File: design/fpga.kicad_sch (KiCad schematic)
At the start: 80 parts, among them J7 DEBUG_FPGA_GPIO, J8 DIGILENT_JTAG_HS2_01X06, SW1 RST, SW2 PROG, U13 XC7S15-FTGB196, U14 IS25LP064A-JKx

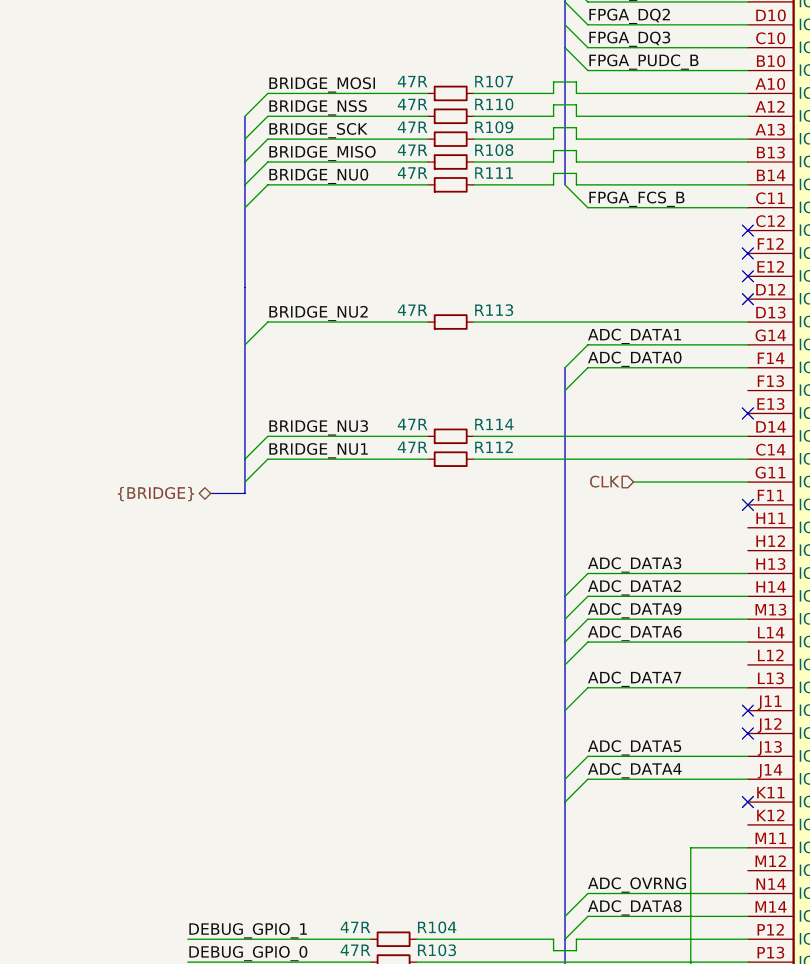
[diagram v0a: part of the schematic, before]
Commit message: Small layout update
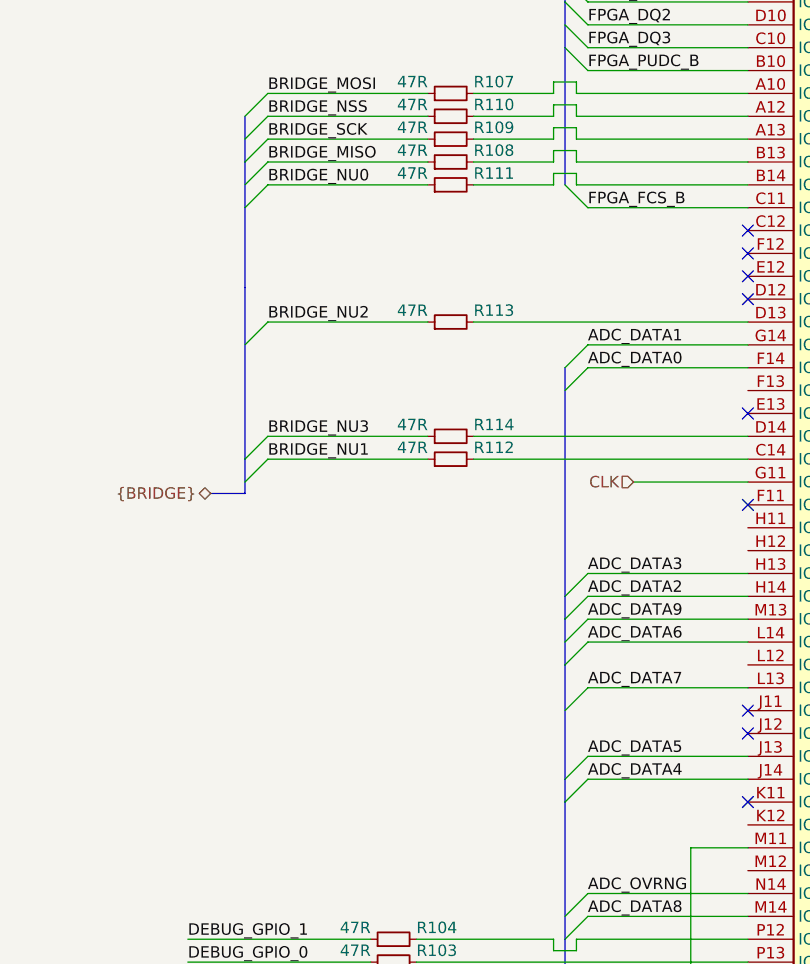
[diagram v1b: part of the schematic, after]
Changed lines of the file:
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@@
   (bus (pts (xy 125.73 85.09) (xy 129.54 85.09)))
   (bus (pts (xy 129.54 43.18) (xy 129.54 48.26)))
-  (bus (pts (xy 129.54 48.26) (xy 129.54 50.8)))
-  (bus (pts (xy 129.54 50.8) (xy 129.54 62.23)))
+  (bus (pts (xy 129.54 48.26) (xy 129.54 53.34)))
+  (bus (pts (xy 129.54 53.34) (xy 129.54 62.23)))
   (bus (pts (xy 129.54 62.23) (xy 129.54 81.28)))
   (bus (pts (xy 129.54 81.28) (xy 129.54 85.09)))
@@
   (bus (pts (xy 165.1 35.56) (xy 165.1 50.8)))
   (bus (pts (xy 165.1 71.12) (xy 165.1 96.52)))
-  (bus (pts (xy 165.1 96.52) (xy 165.1 101.6)))
-  (bus (pts (xy 165.1 101.6) (xy 165.1 109.22)))
-  (bus (pts (xy 165.1 109.22) (xy 165.1 119.38)))
+  (bus (pts (xy 165.1 96.52) (xy 165.1 99.06)))
+  (bus (pts (xy 165.1 99.06) (xy 165.1 104.14)))
+  (bus (pts (xy 165.1 104.14) (xy 165.1 116.84)))
+  (bus (pts (xy 165.1 116.84) (xy 165.1 119.38)))
   (bus (pts (xy 165.1 119.38) (xy 165.1 134.62)))
   (bus (pts (xy 165.1 134.62) (xy 165.1 151.13)))
